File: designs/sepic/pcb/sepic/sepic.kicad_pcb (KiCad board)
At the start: 2 copper layers, 22 parts, among them J2 output, J3 pwm, Q1 irfz44n, U1 INA240A1D, U2 INA240A1D, U3 TC4422

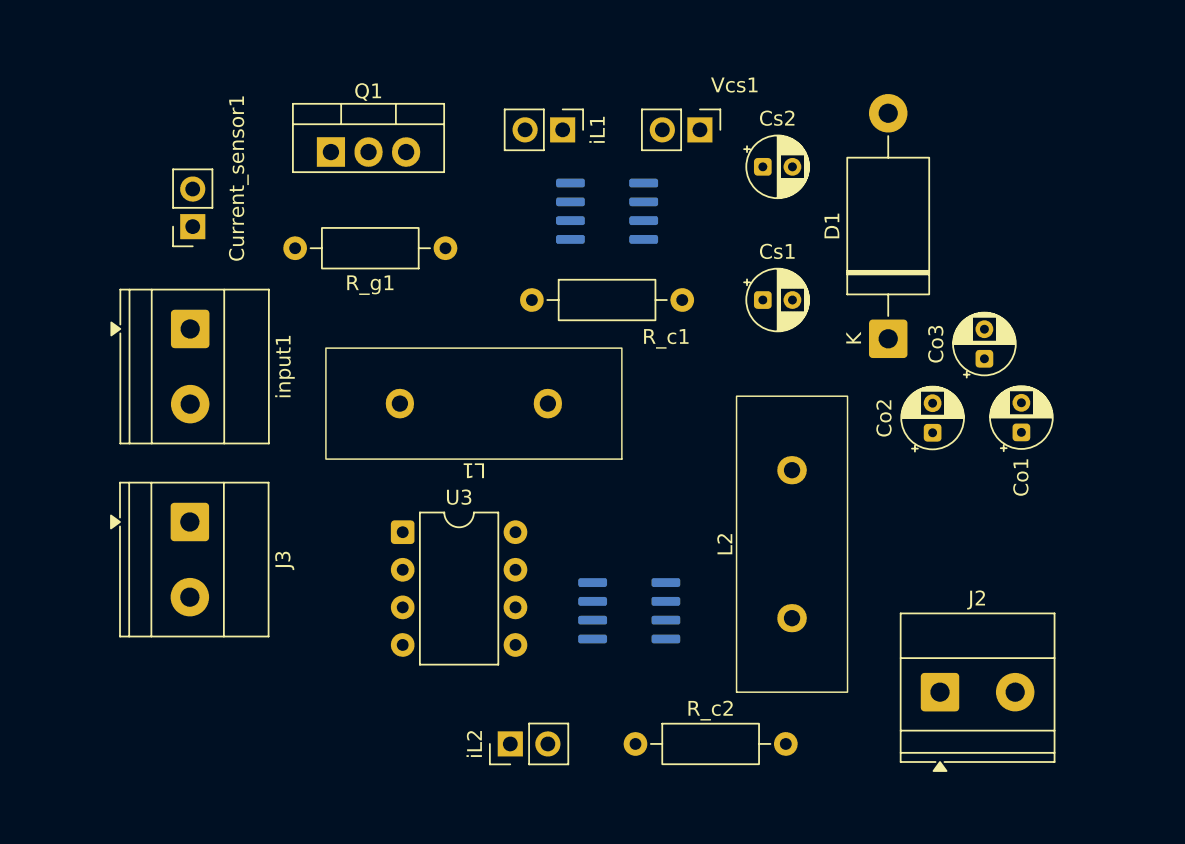
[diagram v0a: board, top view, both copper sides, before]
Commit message: pcb
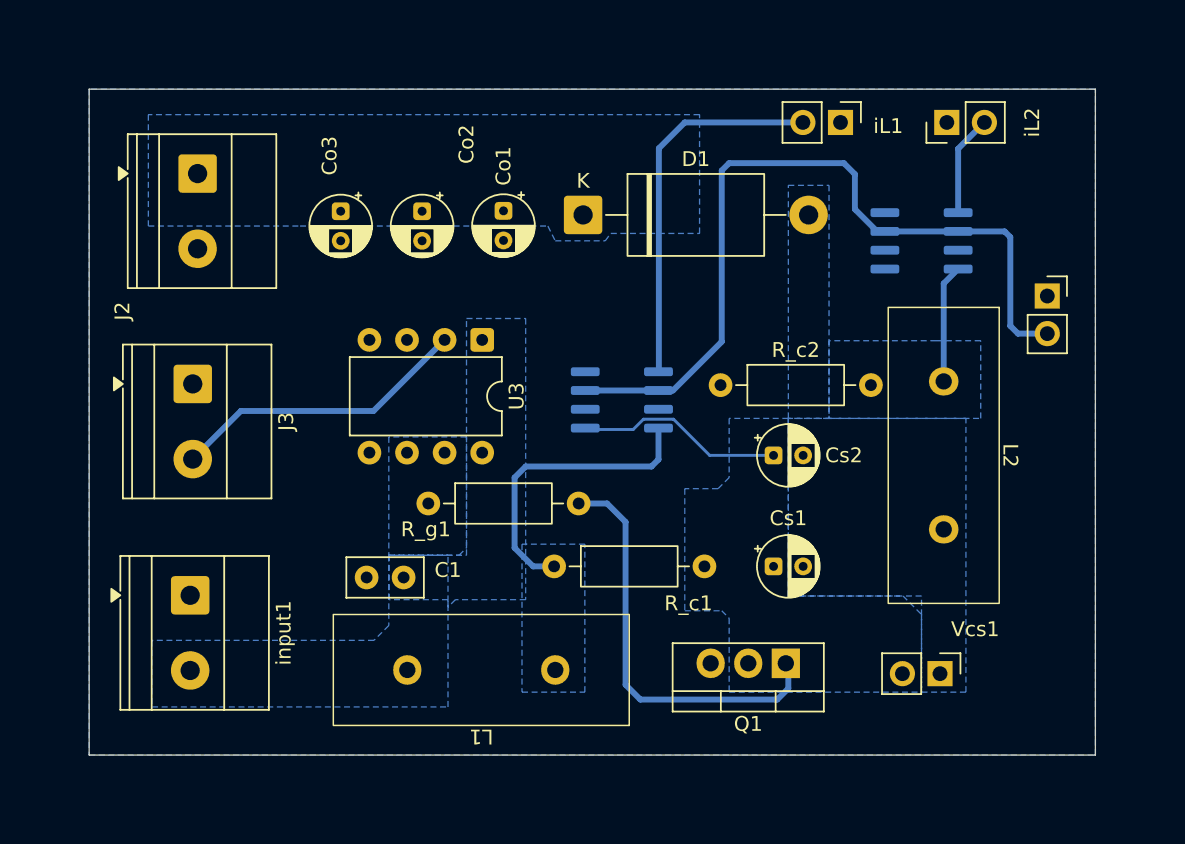
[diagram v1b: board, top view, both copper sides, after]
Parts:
- added C1: 2.2u, Capacitor_THT:C_Disc_D5.0mm_W2.5mm_P2.50mm, F.Cu at (103.2, 118.8)
- R_g1: value 10m -> 10
- moved J2 61.2 mm to (89.3, 91.5), turned to -90 degrees
- moved Current_sensor1 57.9 mm to (146.8, 99.7), turned to 0 degrees
- moved iL2 51.3 mm to (140.0, 88.0)
- moved Q1 46.2 mm to (129.1, 124.5), turned to 180 degrees
- moved Co3 44.6 mm to (99.0, 94.0), turned to -90 degrees
- moved Vcs1 40.2 mm to (139.5, 125.2)
- moved Co1 38.1 mm to (110.0, 94.0), turned to -90 degrees
- moved Co2 37.6 mm to (104.5, 94.0), turned to -90 degrees
- moved U2 31.9 mm to (138.2, 96.0), turned to 0 degrees
- moved R_c2 24.9 mm to (124.7, 105.8)
- moved D1 22.3 mm to (115.4, 94.2), turned to 0 degrees
- moved Cs2 19.5 mm to (128.2, 110.5)
- moved iL1 18.8 mm to (132.8, 88.0)
- moved R_c1 18.1 mm to (113.4, 118.0)
- moved Cs1 18.0 mm to (128.2, 118.0)
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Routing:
- net Net-(Current_sensor1-Pin_2): track 0.00 -> 54.0 mm
- net Net-(Q1-G): track 0.00 -> 28.2 mm
- net Net-(iL1-Pin_2): track 0.00 -> 25.6 mm
- net Net-(J3-Pin_2): track 0.00 -> 20.4 mm
- net /R_cp: track 0.00 -> 20.3 mm
- net /R_cn: track 0.00 -> 14.1 mm
- net /R_c2n: track 0.00 -> 8.00 mm
- net Net-(iL2-Pin_2): track 0.00 -> 6.83 mm
- added copper zone on B.Cu, net /R_c2n
- added copper zone on B.Cu, net /R_cn
- added copper zone on B.Cu, net /R_cp
- added copper zone on B.Cu, net /Vo
- added copper zone on B.Cu, net /pwm
- added copper zone on B.Cu, net GND
- added copper zone on B.Cu, net Net-(D1-A)
- added copper zone on B.Cu, net Net-(input1-Pin_2)
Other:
- board outline added: 68 x 45 mm

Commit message: thinkpad transpport
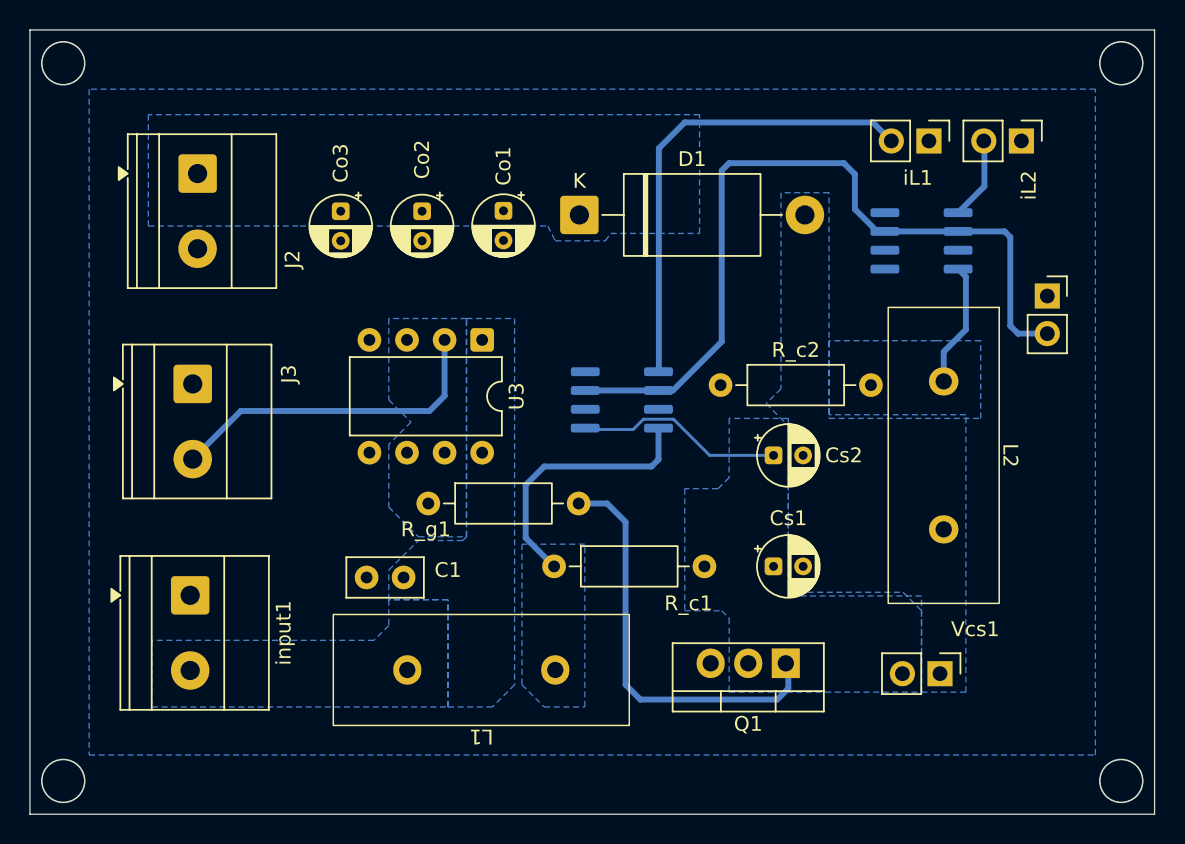
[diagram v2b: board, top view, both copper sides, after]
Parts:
- moved iL1 6.10 mm to (138.8, 89.2)
- moved iL2 5.19 mm to (145.0, 89.2), turned to -90 degrees
- moved D1 0.25 mm to (115.1, 94.2)
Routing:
- net Net-(iL1-Pin_2): track 25.6 -> 32.1 mm
- net Net-(J3-Pin_2): track 20.4 -> 22.6 mm
- net /R_cp: track 20.3 -> 18.1 mm
- net Net-(iL2-Pin_2): track 6.83 -> 5.58 mm
- net (no net): vias 0 -> 4
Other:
- board size 68 x 45 mm -> 76 x 53 mm
